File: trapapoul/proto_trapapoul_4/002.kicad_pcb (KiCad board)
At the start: 2 copper layers, 110 x 50 mm, 116 parts, among them J101 HEADER_3x2, J401 HEADER_2, J402 HEADER_2, J403 HEADER_2, J410 HEADER_4, J730 HEADER_2, J801 HEADER_1, J802 HEADER_1, J901 HEADER_6, J902 HEADER_6, Q811 PBSS4320, Q812 PBSS5350, Q821 PBSS4320, Q822 PBSS5350, Q900 PBSS4320, U100 ATMEGA328P-A, U201 MCP7940, U500 MIC5205, U510 MIC5205, U520 MIC5205, U601 A3144, U602 A3144, U603 A3144, U604 A3144, U715 TLV431-DBZ, U830 MCP601-SOT, U900 PCF8574, X104 16M, X201 32.768K

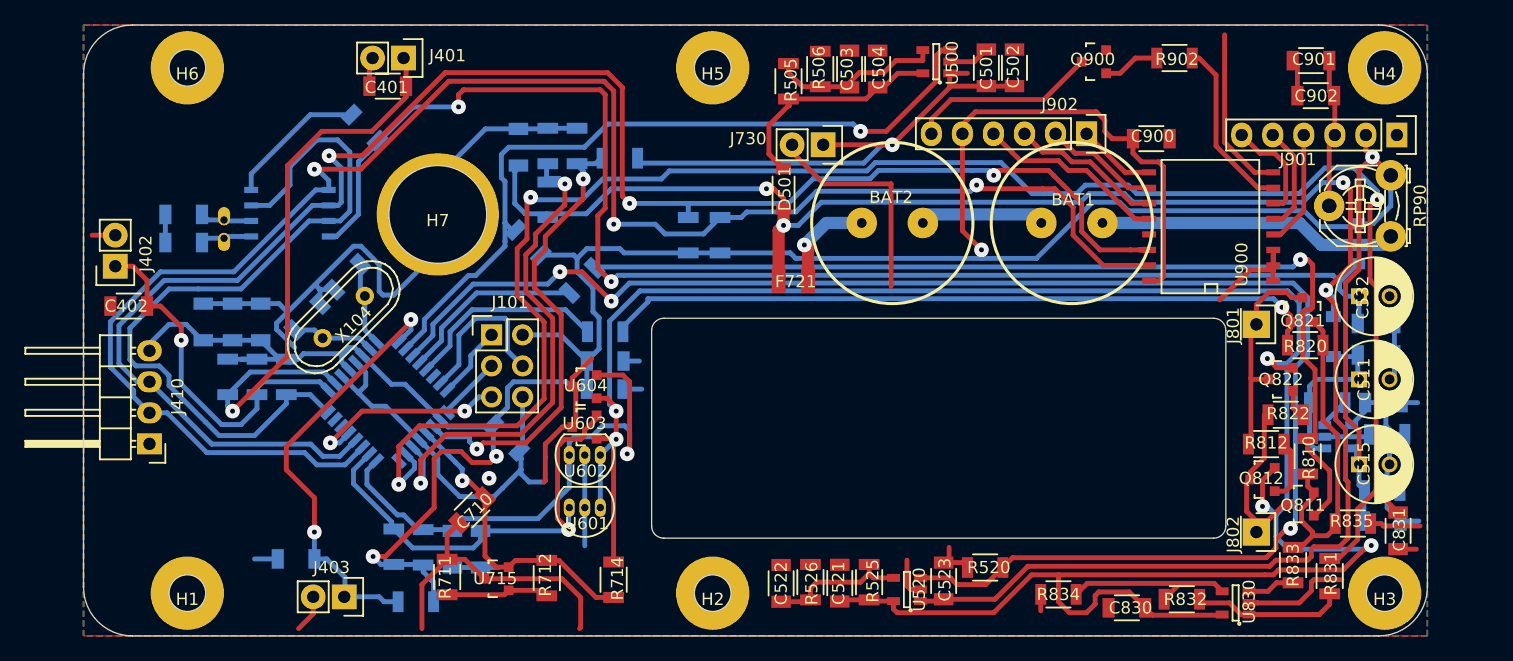
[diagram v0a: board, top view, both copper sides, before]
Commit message: prototrapapoul4 un peu retouché
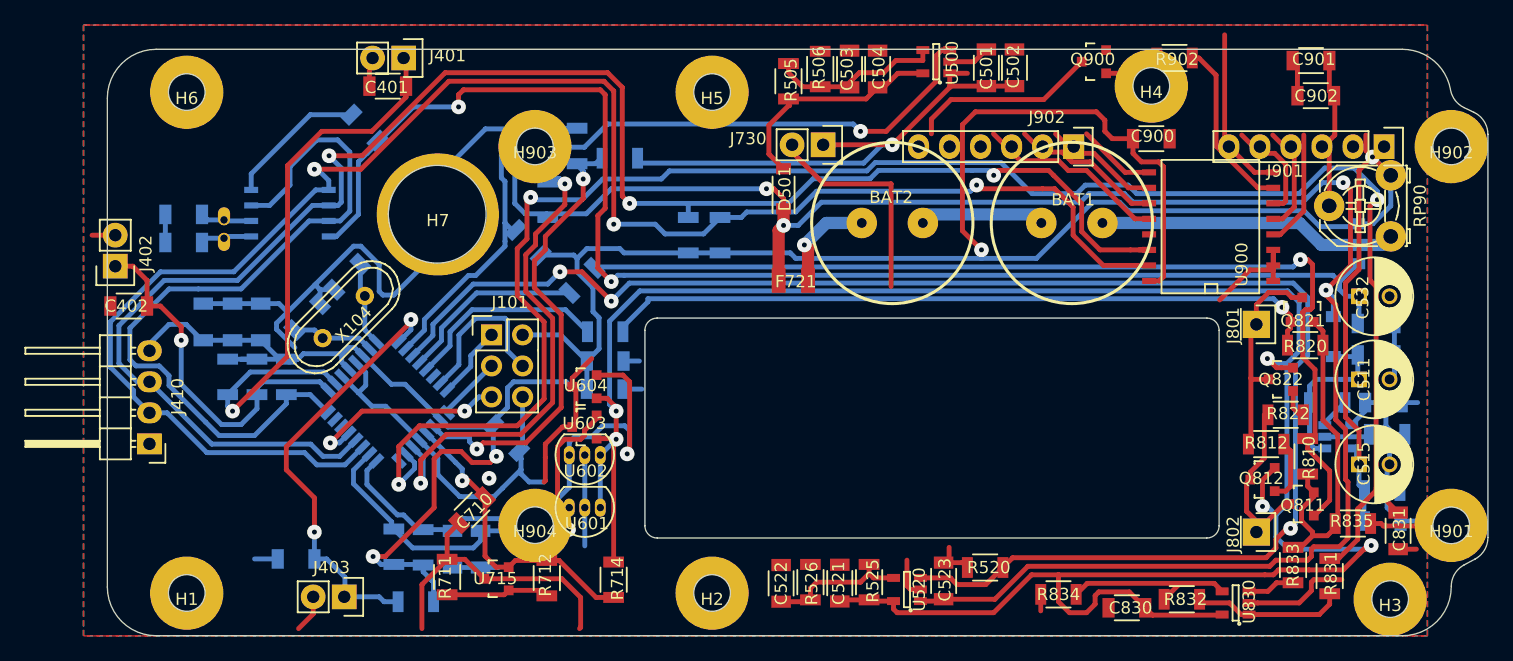
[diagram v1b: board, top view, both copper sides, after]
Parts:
- added H901: hole, gdi:3mm_screw, F.Cu at (211.9, 91.0)
- added H902: hole, gdi:3mm_screw, F.Cu at (211.9, 60.0)
- added H903: hole, gdi:3mm_screw, F.Cu at (136.9, 60.0)
- added H904: hole, gdi:3mm_screw, F.Cu at (136.9, 91.0)
- moved H4 19.2 mm to (187.4, 55.0)
- moved H5 2.00 mm to (151.4, 55.5)
- moved H6 2.00 mm to (108.5, 55.5)
- moved J902 1.48 mm to (181.1, 60.0)
- moved J901 1.42 mm to (206.4, 60.0)
- moved H3 0.67 mm to (206.9, 97.0)
- moved H2 0.05 mm to (151.4, 96.5)
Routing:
- net GND: track 273.6 -> 295.2 mm
- net quadB: track 42.1 -> 32.5 mm
- net quadA: track 38.1 -> 30.8 mm, vias 1 -> 0
- net Net-(Q900-Pad1): track 4.67 -> 1.15 mm
- net M_bat: track 41.1 -> 39.9 mm
- net (no net): vias 0 -> 1
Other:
- board size 110 x 50 mm -> 113 x 48 mm
